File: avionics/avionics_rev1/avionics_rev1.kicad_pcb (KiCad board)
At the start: 2 copper layers, 80 x 25 mm, 47 parts, among them U1 LMR604065SRAKRQ1, U10 LSM6DSV32XTR, U11 MAX-M10S-00B, U2 STM32G474RETx, U8 LPS22DFTR, U9 ADXL375BCCZ-RL7

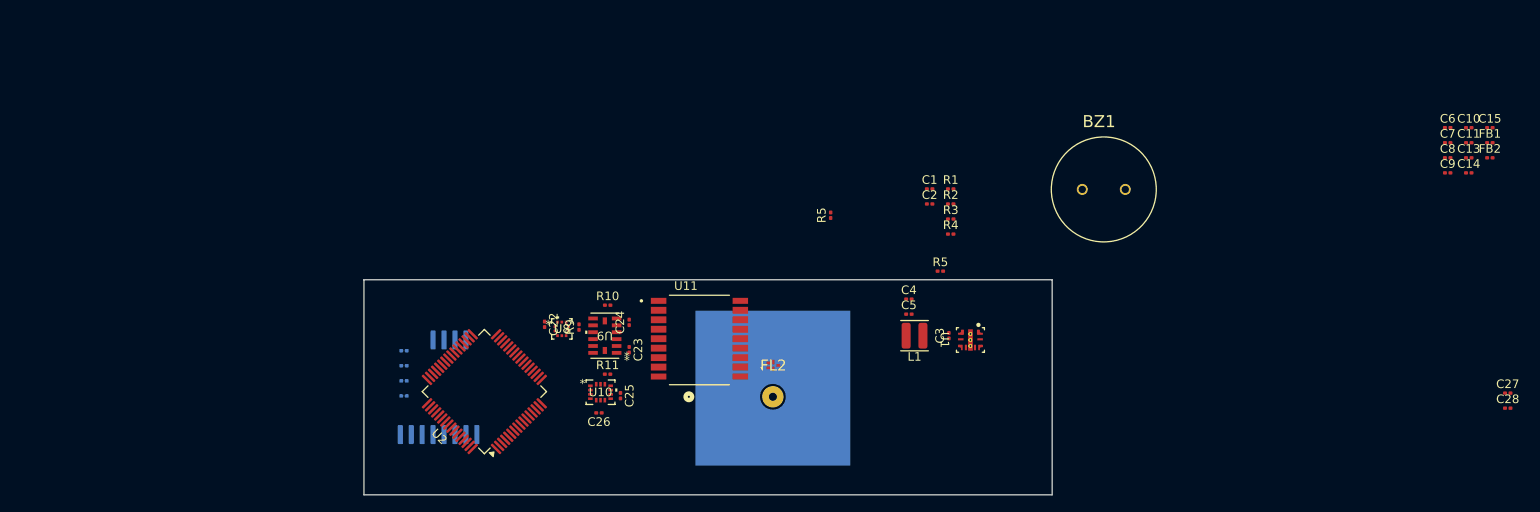
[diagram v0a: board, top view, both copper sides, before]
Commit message: layout 1
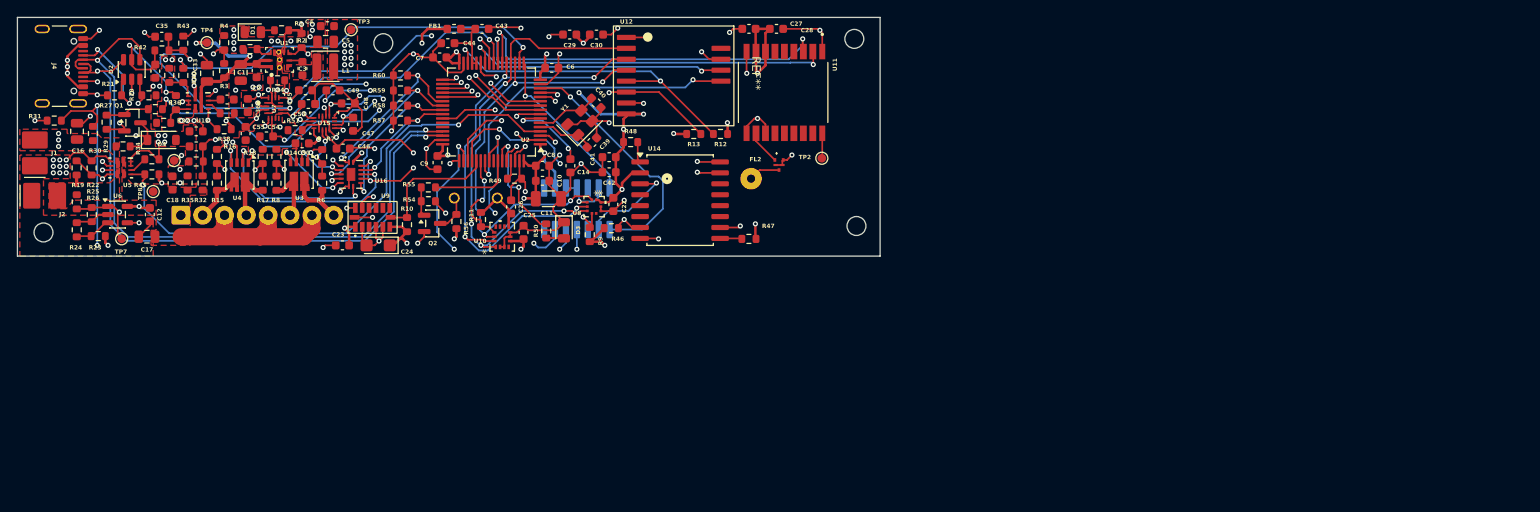
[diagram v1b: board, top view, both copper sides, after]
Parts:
- removed C13: 0.1uF, Capacitor_SMD:C_0201_0603Metric
- removed C15: 1uF, Capacitor_SMD:C_0201_0603Metric
- removed FB2: 600R@100MHz, Capacitor_SMD:C_0201_0603Metric
- removed the R5 at (167.0, 79.0)
- removed the R5 at (154.2, 72.5)
- added C12: 100n, Capacitor_SMD:C_0603_1608Metric, F.Cu at (75.1, 72.4)
- added C16: 10u, Capacitor_SMD:C_0805_2012Metric, F.Cu at (66.6, 62.8)
- added C17: 10u, Capacitor_SMD:C_0805_2012Metric, F.Cu at (74.8, 75.0)
- added C18: 100n, Capacitor_SMD:C_0603_1608Metric, F.Cu at (77.8, 68.8)
- added C19: 10n, Capacitor_SMD:C_0603_1608Metric, F.Cu at (80.5, 64.5)
- added C31: 1u, Capacitor_SMD:C_0603_1608Metric, F.Cu at (80.5, 62.8)
- added C33: 10u, Capacitor_SMD:C_0805_2012Metric, F.Cu at (81.8, 56.0)
- added C34: 100n, Capacitor_SMD:C_0603_1608Metric, F.Cu at (84.1, 59.0)
- added C35: 10n, Capacitor_SMD:C_0603_1608Metric, F.Cu at (76.5, 51.8)
- added C36: 100n, Capacitor_SMD:C_0603_1608Metric, F.Cu at (86.5, 59.8)
- added C38: 100n, Capacitor_SMD:C_0603_1608Metric, F.Cu at (75.8, 55.8)
- added C39: 10p, Capacitor_SMD:C_0603_1608Metric, F.Cu at (126.5, 64.0)
- added C40: 10p, Capacitor_SMD:C_0603_1608Metric, F.Cu at (127.0, 59.5)
- added C41: 100n, Capacitor_SMD:C_0603_1608Metric, F.Cu at (128.5, 65.8)
- added C42: 1u, Capacitor_SMD:C_0603_1608Metric, F.Cu at (128.5, 67.5)
- added C43: 1u, Capacitor_SMD:C_0603_1608Metric, F.Cu at (113.7, 50.8)
- added C44: 100n, Capacitor_SMD:C_0603_1608Metric, F.Cu at (109.8, 52.5)
- added C45: 10n, Capacitor_SMD:C_0603_1608Metric, F.Cu at (93.2, 58.0)
- added C46: 10n, Capacitor_SMD:C_0603_1608Metric, F.Cu at (97.6, 64.8)
- added C47: 10n, Capacitor_SMD:C_0603_1608Metric, F.Cu at (98.7, 61.9)
- added C48: 10n, Capacitor_SMD:C_0603_1608Metric, F.Cu at (98.2, 59.5)
- added C49: 10n, Capacitor_SMD:C_0603_1608Metric, F.Cu at (96.4, 58.0)
- added C50: 100n, Capacitor_SMD:C_0603_1608Metric, F.Cu at (92.8, 64.1)
- added C53: 10n, Capacitor_SMD:C_0603_1608Metric, F.Cu at (93.5, 59.6)
- added C54: 10n, Capacitor_SMD:C_0603_1608Metric, F.Cu at (88.7, 63.3)
- added C55: 10n, Capacitor_SMD:C_0603_1608Metric, F.Cu at (86.2, 63.0)
- added D1: LTST-C170GKT, avionics_footprints:LTST_C170GKT_0805, F.Cu at (87.1, 51.2)
- added D2: USBLC6-4SC6, avionics_footprints:USBLC6_4SC6_SOT23_6, F.Cu at (73.0, 55.6)
- added D3: LTST-C170GKT, avionics_footprints:LTST_C170GKT_0805, F.Cu at (123.2, 74.2)
- added D4: BZT52C4V7-E3-08, avionics_footprints:BZT52C4V7_E3_08_SOD123, F.Cu at (76.5, 63.8)
- added H1: MountingHole, MountingHole:MountingHole_2.2mm_M2, F.Cu at (102.2, 52.5)
- added H2: MountingHole, MountingHole:MountingHole_2.2mm_M2, F.Cu at (157.0, 52.0)
- added H3: MountingHole, MountingHole:MountingHole_2.2mm_M2, F.Cu at (157.2, 73.8)
- added H4: MountingHole, MountingHole:MountingHole_2.2mm_M2, F.Cu at (62.8, 74.5)
- added J1: Wire_Solder_Pads, avionics_footprints:WireSolderPads_1x02_3x2mm_P4mm, F.Cu at (61.7, 66.2)
- added J2: Wire_Solder_Pads, avionics_footprints:WireSolderPads_1x02_3x2mm_P4mm, F.Cu at (61.9, 70.2)
- added J3: 1725711, avionics_footprints:Phoenix_1725711_MPT_0.5_8_2.54, B.Cu at (78.7, 72.5)
- added J4: USB4105-GF-A, Connector_USB:USB_C_Receptacle_GCT_USB4105-xx-A_16P_TopMnt_Horizontal, F.Cu at (63.7, 55.2)
- added J5: FTSH-107-01-L-DV-K, avionics_footprints:FTSH-107-01-L-DV-K_STDC14, B.Cu at (124.8, 71.8)
- added Q1: DMN2056U-7, avionics_footprints:DMN2056U_7_SOT23, F.Cu at (73.1, 61.8)
- added Q2: DMN2056U-7, avionics_footprints:DMN2056U_7_SOT23, F.Cu at (107.9, 73.5)
- added R14: 18k, Resistor_SMD:R_0603_1608Metric, F.Cu at (89.8, 65.7)
- added R15: 100k, Resistor_SMD:R_0603_1608Metric, F.Cu at (82.9, 68.8)
- added R16: 18k, Resistor_SMD:R_0603_1608Metric, F.Cu at (82.9, 65.7)
- added R17: 100k, Resistor_SMD:R_0603_1608Metric, F.Cu at (88.2, 68.8)
- added R18: 18k, Resistor_SMD:R_0603_1608Metric, F.Cu at (88.2, 65.7)
- added R19: 20k, Resistor_SMD:R_0603_1608Metric, F.Cu at (66.6, 67.0)
- added R20: 5.1k, Resistor_SMD:R_0603_1608Metric, F.Cu at (75.0, 58.6)
- added R21: 5.1k, Resistor_SMD:R_0603_1608Metric, F.Cu at (71.0, 58.6)
- added R22: 10k, Resistor_SMD:R_0603_1608Metric, F.Cu at (68.3, 67.0)
- added R23: 18.2k, Resistor_SMD:R_0603_1608Metric, F.Cu at (69.1, 74.9)
- added R24: 10k, Resistor_SMD:R_0603_1608Metric, F.Cu at (66.6, 74.2)
- added R25: 47k, Resistor_SMD:R_0603_1608Metric, F.Cu at (66.6, 70.9)
- added R26: 47k, Resistor_SMD:R_0603_1608Metric, F.Cu at (68.4, 72.4)
- added R27: 100k, Resistor_SMD:R_0603_1608Metric, F.Cu at (70.1, 61.7)
- added R28: 1k, Resistor_SMD:R_0603_1608Metric, F.Cu at (75.8, 60.2)
- added R29: 10k, Resistor_SMD:R_0603_1608Metric, F.Cu at (72.0, 64.5)
- added R30: 49.9k, Resistor_SMD:R_0603_1608Metric, F.Cu at (68.5, 63.0)
- added R31: 10k, Resistor_SMD:R_0603_1608Metric, F.Cu at (64.0, 61.5)
- added R32: 49.9k, Resistor_SMD:R_0603_1608Metric, F.Cu at (81.2, 68.8)
- added R33: 10k, Resistor_SMD:R_0603_1608Metric, F.Cu at (80.5, 66.2)
- added R34: 22.1k, Resistor_SMD:R_0603_1608Metric, F.Cu at (75.3, 66.0)
- added R35: 47k, Resistor_SMD:R_0603_1608Metric, F.Cu at (79.5, 68.8)
- added R36: 15k, Resistor_SMD:R_0603_1608Metric, F.Cu at (78.1, 59.4)
- added R37: 10k, Resistor_SMD:R_0603_1608Metric, F.Cu at (76.7, 61.8)
- added R38: 10k, Resistor_SMD:R_0603_1608Metric, F.Cu at (83.8, 62.5)
- added R39: 80.6k, Resistor_SMD:R_0603_1608Metric, F.Cu at (84.1, 60.6)
- added R40: 1k, Resistor_SMD:R_0603_1608Metric, F.Cu at (79.0, 56.2)
- added R41: 100k, Resistor_SMD:R_0603_1608Metric, F.Cu at (77.4, 56.2)
- added R42: 49.9k, Resistor_SMD:R_0603_1608Metric, F.Cu at (76.5, 53.3)
- added R43: 10k, Resistor_SMD:R_0603_1608Metric, F.Cu at (79.0, 52.5)
- added R44: 10k, Resistor_SMD:R_0603_1608Metric, F.Cu at (90.0, 56.8)
- added R45: 10k, Resistor_SMD:R_0603_1608Metric, F.Cu at (75.3, 67.8)
- added R46: 10k, Resistor_SMD:R_0603_1608Metric, F.Cu at (128.8, 74.0)
- added R47: 10k, Resistor_SMD:R_0603_1608Metric, F.Cu at (144.8, 75.2)
- added R48: 10k, Resistor_SMD:R_0603_1608Metric, F.Cu at (131.0, 64.0)
- added R49: 10k, Resistor_SMD:R_0603_1608Metric, F.Cu at (117.5, 68.2)
- added R5: 120, Resistor_SMD:R_0603_1608Metric, F.Cu at (90.4, 51.0)
- added R50: 1k, Resistor_SMD:R_0603_1608Metric, F.Cu at (121.2, 74.3)
- added R51: 10k, Resistor_SMD:R_0603_1608Metric, F.Cu at (92.0, 62.6)
- added R54: 1k, Resistor_SMD:R_0603_1608Metric, F.Cu at (107.5, 69.3)
- added R55: 10k, Resistor_SMD:R_0603_1608Metric, F.Cu at (107.5, 70.9)
- added R56: 1k, Resistor_SMD:R_0603_1608Metric, F.Cu at (110.7, 73.2)
- added R57: 10k, Resistor_SMD:R_0603_1608Metric, F.Cu at (104.2, 61.5)
- added R58: 10k, Resistor_SMD:R_0603_1608Metric, F.Cu at (104.2, 59.8)
- added R59: 10k, Resistor_SMD:R_0603_1608Metric, F.Cu at (104.2, 58.0)
- added R6: 100k, Resistor_SMD:R_0603_1608Metric, F.Cu at (95.1, 68.8)
- added R60: 10k, Resistor_SMD:R_0603_1608Metric, F.Cu at (104.2, 56.2)
- added R7: 18k, Resistor_SMD:R_0603_1608Metric, F.Cu at (95.1, 65.7)
- added R8: 100k, Resistor_SMD:R_0603_1608Metric, F.Cu at (89.8, 68.8)
- added TP2: TestPoint, TestPoint:TestPoint_Pad_D1.0mm, F.Cu at (153.2, 65.9)
- added TP3: TestPoint, TestPoint:TestPoint_Pad_D1.0mm, F.Cu at (98.5, 50.9)
- added TP4: TestPoint, TestPoint:TestPoint_Pad_D1.0mm, F.Cu at (81.8, 52.4)
- added TP7: TestPoint, TestPoint:TestPoint_Pad_D1.0mm, F.Cu at (71.8, 75.2)
- added TP8: TestPoint, TestPoint:TestPoint_Pad_D1.0mm, F.Cu at (75.5, 69.8)
- added TP9: TestPoint, TestPoint:TestPoint_Pad_D1.0mm, F.Cu at (77.9, 66.1)
- added U13: TPS2121RUXR, avionics_footprints:TPS2121RUXR_RUX12, F.Cu at (80.8, 59.4)
- added U14: W25Q512JVFIM, avionics_footprints:W25Q512JVFIM_SOIC16W, F.Cu at (136.8, 70.8)
- added U15: TMUX1511RSVR, avionics_footprints:TMUX1511RSVR_RSV16, F.Cu at (95.4, 61.8)
- added U16: SN74LVC08AWBQARQ1, avionics_footprints:SN74LVC08AWBQARQ1_BQA14, F.Cu at (98.5, 67.8)
- added U3: SIS932EDN-T1-GE3, avionics_footprints:SIS932EDN_PowerPAK1212_8_Dual, F.Cu at (92.5, 67.7)
- added U4: SIS932EDN-T1-GE3, avionics_footprints:SIS932EDN_PowerPAK1212_8_Dual, F.Cu at (85.6, 67.8)
- added U5: TPS2121RUXR, avionics_footprints:TPS2121RUXR_RUX12, F.Cu at (71.8, 67.0)
- added U6: TLV7041DBVR, avionics_footprints:TLV7041DBVR_SOT23_5, F.Cu at (71.4, 72.4)
- added U7: TMUX1511RSVR, avionics_footprints:TMUX1511RSVR_RSV16, F.Cu at (89.5, 60.0)
- added Y1: 16MHz / CL10pF, avionics_footprints:ABM8_3.2x2.5mm, F.Cu at (125.1, 61.8)
- AE2: value Antenna -> GP.1575.18.4.A.02
- BZ1: value Buzzer -> PS1240P02BT; moved to B.Cu
- C1: value 4.7uF -> 4.7u; footprint Capacitor_SMD:C_0201_0603Metric -> Capacitor_SMD:C_0805_2012Metric
- C10, C28: value 1uF -> 1u; footprint Capacitor_SMD:C_0201_0603Metric -> Capacitor_SMD:C_0603_1608Metric
- C11: value 47uF -> 47u; footprint Capacitor_SMD:C_0201_0603Metric -> Capacitor_SMD:C_1206_3216Metric
- C14, C2, C22, C23, C25, C26, C27, C3, C6, C7, C8, C9: value 0.1uF -> 100n; footprint Capacitor_SMD:C_0201_0603Metric -> Capacitor_SMD:C_0603_1608Metric
- C24: value 1uF -> 1u; footprint Capacitor_SMD:C_0201_0603Metric -> avionics_footprints:TAJA105K016RNJ_3216_18
- C29: value 0.1uF -> 100n; footprint Capacitor_SMD:C_0201_0603Metric -> Capacitor_SMD:C_0603_1608Metric; moved to F.Cu
- C30: value 1uF -> 1u; footprint Capacitor_SMD:C_0201_0603Metric -> Capacitor_SMD:C_0603_1608Metric; moved to F.Cu
- C4: value 4.7uF -> 4.7u; footprint Capacitor_SMD:C_0201_0603Metric -> Capacitor_SMD:C_0603_1608Metric
- C5: value 10uF -> 10u; footprint Capacitor_SMD:C_0201_0603Metric -> Capacitor_SMD:C_0805_2012Metric
- FB1: footprint Capacitor_SMD:C_0201_0603Metric -> Inductor_SMD:L_0603_1608Metric
- R1: value 15.2ohm -> 15.2k; footprint Resistor_SMD:R_0201_0603Metric -> Resistor_SMD:R_0603_1608Metric
- R10: value 47k -> 10k; footprint Resistor_SMD:R_0201_0603Metric -> Resistor_SMD:R_0603_1608Metric
- R11, R2, R3, R4, R9: footprint Resistor_SMD:R_0201_0603Metric -> Resistor_SMD:R_0603_1608Metric
- R12, R13: footprint Resistor_SMD:R_0201_0603Metric -> Resistor_SMD:R_0603_1608Metric; moved to F.Cu
- U1: value LMR604065SRAKRQ1 -> LMR604063SBRAKRQ1; footprint avionics_footprints:RAK0009A-MFG -> avionics_footprints:LMR604063SBRAKRQ1_RAK9
- U12: value ~ -> Wio-SX1262; moved to F.Cu
- U2: value STM32G474RETx -> STM32G474RET6
- moved FB1 121.1 mm to (110.5, 50.8)
- moved C7 117.6 mm to (108.8, 54.2), turned to 180 degrees
- moved C9 117.4 mm to (108.5, 66.4), turned to -90 degrees
- moved C10 107.9 mm to (120.8, 68.5)
- moved C11 107.2 mm to (121.4, 70.6)
- moved C8 105.2 mm to (120.8, 66.7)
- moved C14 104.4 mm to (124.0, 66.8), turned to -90 degrees
- moved C6 104.4 mm to (121.8, 55.4)
- moved C27 97.8 mm to (144.8, 50.8)
- moved C28 95.8 mm to (148.0, 50.8), turned to 180 degrees
- moved R4 87.3 mm to (83.8, 52.4), turned to -90 degrees
- moved U1 86.7 mm to (90.2, 54.4), turned to 90 degrees
- moved R3 86.2 mm to (83.8, 55.7), turned to -90 degrees
- moved R1 83.1 mm to (86.8, 53.2)
- moved C3 81.3 mm to (92.9, 55.4), turned to -90 degrees
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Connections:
- net SENS_BATT renamed SENS_LOGIC_VIN
- net VIN_BATT renamed VIN_LOGIC
- BZ1 pad 1: unconnected-(BZ1-+-Pad1) -> +3.3V
- BZ1 pad 2: unconnected-(BZ1---Pad2) -> Net-(BZ1--)
- C14 pad 1: GND -> /MCU/NRST
- C14 pad 2: +3.3V -> GND
- C24 pad 1: GND -> +3.3V
- C24 pad 2: +3.3V -> GND
- C27 pad 1: Net-(C27-Pad1) -> GND
- C28 pad 1: Net-(C27-Pad1) -> GND
- C30 pad 1: GND -> +3.3V
- C30 pad 2: +3.3V -> GND
- C6 pad 1: GND -> +3.3V
- C6 pad 2: +3.3V -> GND
- C7 pad 1: GND -> +3.3V
- C7 pad 2: +3.3V -> GND
- C8 pad 1: GND -> +3.3V
- C8 pad 2: +3.3V -> GND
- FB1 pad 2: Net-(U2-VDDA) -> /MCU/VDDA_FILTERED
- R2 pad 2: PG_SENS -> MCU_PG_SENS
- U1 pad 5: PG_SENS -> MCU_PG_SENS
- U12 pad 2: SPI1_MOSI -> SPI1_MISO
- U12 pad 3: SPI1_MISO -> SPI1_MOSI
- U2 pad 10: unconnected-(U2-PC2-Pad10) -> ADC_PYRO_3
- U2 pad 11: unconnected-(U2-PC3-Pad11) -> ADC_PYRO_4
- U2 pad 12: unconnected-(U2-PA0-Pad12) -> ADC_MAIN
- U2 pad 13: unconnected-(U2-PA1-Pad13) -> ADC_PYRO_POWER
- U2 pad 14: unconnected-(U2-PA2-Pad14) -> /MCU/DEBUG_UART_TX
- U2 pad 17: unconnected-(U2-PA3-Pad17) -> /MCU/DEBUG_UART_RX
- U2 pad 18: unconnected-(U2-PA4-Pad18) -> MCU_SELECT_MAIN
- U2 pad 2: unconnected-(U2-PC13-Pad2) -> MCU_PG_SENS
- U2 pad 24: unconnected-(U2-PB0-Pad24) -> ADC_USB
- U2 pad 25: unconnected-(U2-PB1-Pad25) -> ADC_LOGIC
- U2 pad 26: unconnected-(U2-PB2-Pad26) -> RADIO_BUSY
- U2 pad 28: /MCU/VREF -> /MCU/VDDA_FILTERED
- U2 pad 29: Net-(U2-VDDA) -> /MCU/VDDA_FILTERED
- U2 pad 3: unconnected-(U2-PC14-Pad3) -> LOGIC_PMUX_ST
- U2 pad 30: unconnected-(U2-PB10-Pad30) -> RADIO_REBOOT
- U2 pad 33: unconnected-(U2-PB11-Pad33) -> RADIO_RF_SW
- U2 pad 34: unconnected-(U2-PB12-Pad34) -> /MCU/CS_FLASH
- U2 pad 35: unconnected-(U2-PB13-Pad35) -> /MCU/SPI2_SCK
- U2 pad 36: unconnected-(U2-PB14-Pad36) -> /MCU/SPI2_MISO
- U2 pad 37: unconnected-(U2-PB15-Pad37) -> /MCU/SPI2_MOSI
- U2 pad 38: unconnected-(U2-PC6-Pad38) -> PYRO_1_FIRE
- U2 pad 39: unconnected-(U2-PC7-Pad39) -> PYRO_2_FIRE
- U2 pad 4: unconnected-(U2-PC15-Pad4) -> PYRO_PMUX_ST
- U2 pad 40: unconnected-(U2-PC8-Pad40) -> PYRO_3_FIRE
- U2 pad 41: unconnected-(U2-PC9-Pad41) -> PYRO_4_FIRE
- U2 pad 42: unconnected-(U2-PA8-Pad42) -> CS_RADIO
- U2 pad 45: unconnected-(U2-PA11-Pad45) -> USB_D-
- U2 pad 46: unconnected-(U2-PA12-Pad46) -> USB_D+
- U2 pad 49: unconnected-(U2-PA13-Pad49) -> /MCU/SWDIO
- U2 pad 5: unconnected-(U2-PF0-Pad5) -> /MCU/OSC_IN
- U2 pad 50: unconnected-(U2-PA14-Pad50) -> /MCU/SWCLK
- U2 pad 51: unconnected-(U2-PA15-Pad51) -> GPS_RESET
- U2 pad 52: unconnected-(U2-PC10-Pad52) -> CS_BARO
- U2 pad 53: unconnected-(U2-PC11-Pad53) -> CS_ACCEL
- U2 pad 54: unconnected-(U2-PC12-Pad54) -> CS_IMU
- U2 pad 55: unconnected-(U2-PD2-Pad55) -> RADIO_INT
- U2 pad 56: unconnected-(U2-PB3-Pad56) -> /MCU/SWO
- U2 pad 58: unconnected-(U2-PB5-Pad58) -> /MCU/BUZZER_PWM
- U2 pad 59: unconnected-(U2-PB6-Pad59) -> /MCU/STATUS_LED
- U2 pad 6: unconnected-(U2-PF1-Pad6) -> /MCU/OSC_OUT
- U2 pad 60: unconnected-(U2-PB7-Pad60) -> PYRO_SEL_IN2
- U2 pad 61: unconnected-(U2-PB8-Pad61) -> /MCU/BOOT0
- U2 pad 62: unconnected-(U2-PB9-Pad62) -> SENSE_EN
- U2 pad 7: unconnected-(U2-PG10-Pad7) -> /MCU/NRST
- U2 pad 8: unconnected-(U2-PC0-Pad8) -> ADC_PYRO_1
- U2 pad 9: unconnected-(U2-PC1-Pad9) -> ADC_PYRO_2
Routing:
- net +3.3V: track 0.00 -> 350.0 mm, vias 0 -> 36
- net GND: track 0.00 -> 218.2 mm, vias 0 -> 78
- net USB_D-: track 0.00 -> 79.8 mm, vias 0 -> 2
- net USB_D+: track 0.00 -> 75.2 mm, vias 0 -> 2
- net SPI1_MOSI: track 0.00 -> 74.0 mm, vias 0 -> 5
- net SPI1_MISO: track 0.00 -> 71.2 mm, vias 0 -> 5
- net SPI1_SCK: track 0.00 -> 67.6 mm, vias 0 -> 5
- net PYRO_PMUX_ST: track 0.00 -> 62.6 mm, vias 0 -> 2
- net SENSE_EN: track 0.00 -> 60.0 mm, vias 0 -> 3
- net LOGIC_PMUX_ST: track 0.00 -> 56.1 mm, vias 0 -> 2
- net PYRO_SEL_IN2: track 0.00 -> 55.0 mm, vias 0 -> 3
- net MCU_PG_SENS: track 0.00 -> 53.0 mm, vias 0 -> 7
- net MAIN_BAT_SENS: track 0.00 -> 52.6 mm, vias 0 -> 3
- net ADC_PYRO_POWER: track 0.00 -> 49.4 mm, vias 0 -> 2
- net MCU_SELECT_MAIN: track 0.00 -> 46.4 mm, vias 0 -> 2
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- added copper zone on F.Cu, net +3.3V
- added copper zone on In2.Cu, net +3.3V
- added copper zone on F.Cu, net GND
- added copper zone on In1.Cu, net GND
- added copper zone on F.Cu, net Net-(U1-SW)
- added copper zone on F.Cu, net PYRO_POWER
- added copper zone on F.Cu, net VIN_MAIN_BATT
- added copper zone on F.Cu, net VIN_PYRO_BATT
- added copper zone on F.Cu, net VIN_USB
- added copper zone on In2.Cu, net VIN_USB
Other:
- board size 80 x 25 mm -> 100.3 x 27.7 mm
- copper layers 2 -> 4
